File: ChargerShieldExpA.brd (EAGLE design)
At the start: 160 x 99.1 mm, 101 parts, among them IC1 TL431, IC2 LM324N, Q1 BUZ11, Q2 BD648, Q3 BUZ171, Q4 IRFZ48Z, T1 BC548, X1 +Vin, X2 VCC, X3 Battery

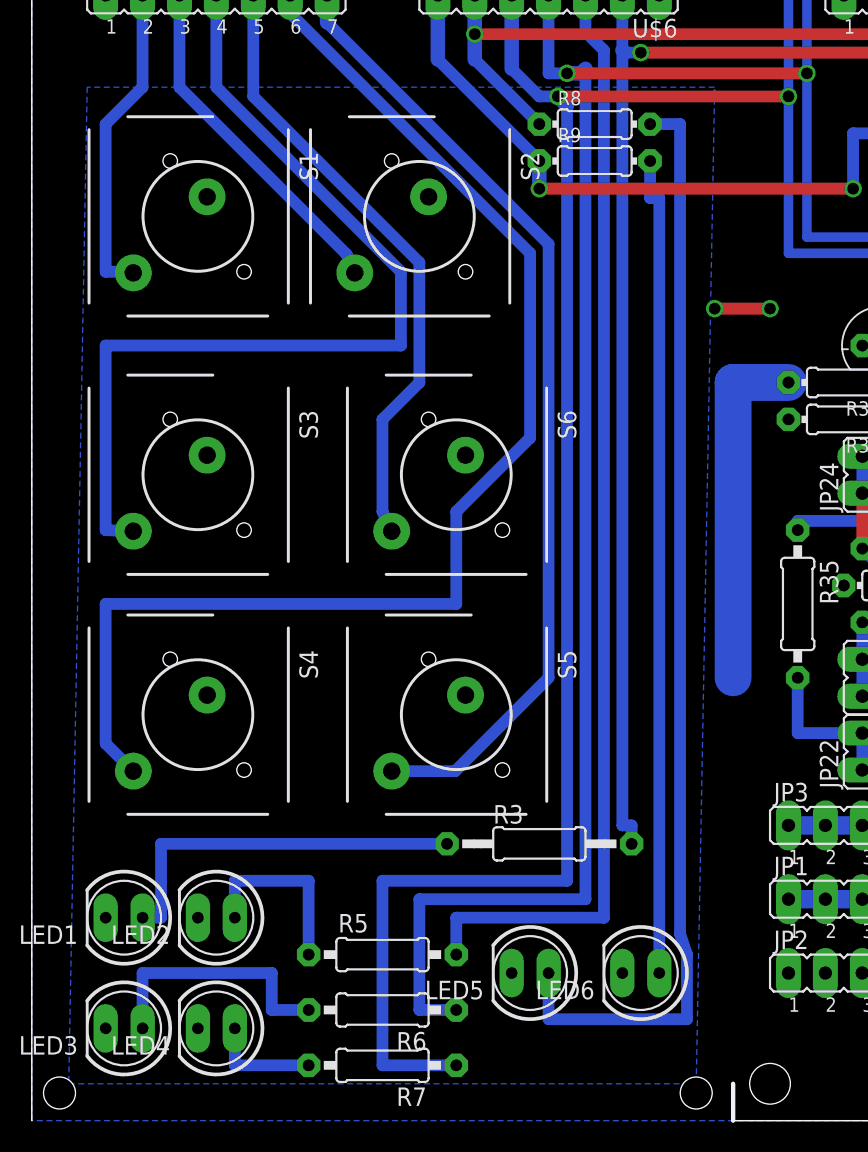
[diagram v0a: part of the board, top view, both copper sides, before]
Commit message: update
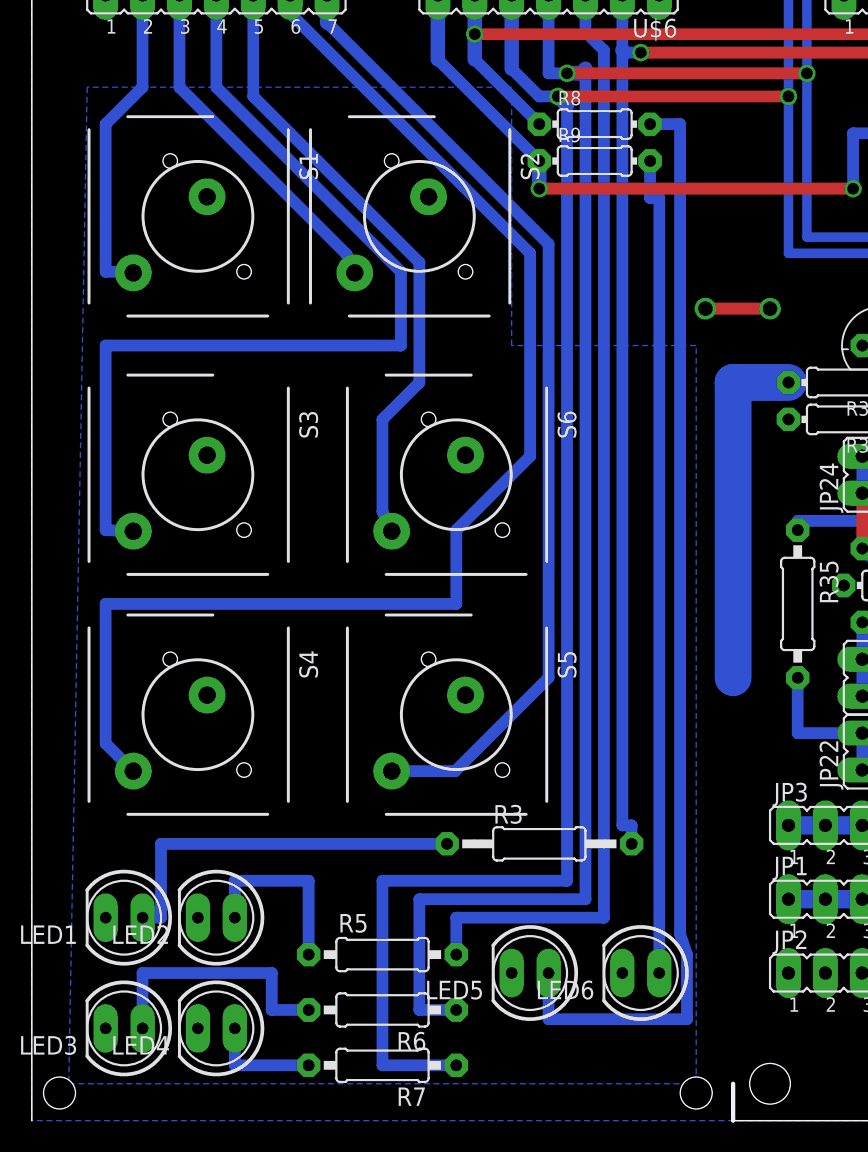
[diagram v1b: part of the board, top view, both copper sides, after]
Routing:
- net GND: track 168.7 -> 169.3 mm
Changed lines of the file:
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@@
 <setting verticaltext="up"/>
 </settings>
-<grid distance="1.27" unitdist="mm" unit="mm" style="lines" multiple="2" display="yes" altdistance="0.15875" altunitdist="mm" altunit="mm"/>
+<grid distance="0.05" unitdist="inch" unit="mm" style="lines" multiple="1" display="yes" altdistance="0.025" altunitdist="inch" altunit="mm"/>
 <layers>
 <layer number="1" name="Top" color="4" fill="1" visible="yes" active="yes"/>
@@
 <wire x1="19.05" y1="11.43" x2="19.05" y2="-3.81" width="0.8128" layer="1" style="shortdash"/>
 <contactref element="JP20" pad="3"/>
-<via x="5.08" y="38.1" extent="1-16" drill="0.8" shape="square"/>
+<via x="5.08" y="38.1" extent="1-16" drill="1" shape="square"/>
 <wire x1="22.86" y1="-7.62" x2="22.86" y2="-11.47" width="1.6764" layer="16"/>
 <wire x1="22.86" y1="-11.47" x2="22.82" y2="-10.16" width="1.6764" layer="16"/>
@@
 <contactref element="S4" pad="1"/>
 <contactref element="S5" pad="1"/>
-<via x="1.27" y="38.1" extent="1-16" drill="0.8" shape="square"/>
-<wire x1="1.27" y1="38.1" x2="5.08" y2="38.1" width="0.8128" layer="1"/>
+<via x="0.635" y="38.1" extent="1-16" drill="1" shape="square"/>
+<wire x1="0.635" y1="38.1" x2="5.08" y2="38.1" width="0.8128" layer="1"/>
 <wire x1="2.54" y1="33.02" x2="2.54" y2="12.7" width="2.54" layer="16"/>
 <wire x1="2.54" y1="33.02" x2="6.35" y2="33.02" width="2.54" layer="16"/>
@@
 <polygon width="1.27" layer="16" isolate="0.6096" orphans="yes">
 <vertex x="0" y="-15.24"/>
-<vertex x="1.27" y="53.34"/>
+<vertex x="0" y="35.56"/>
+<vertex x="-12.7" y="35.56"/>
+<vertex x="-12.7" y="53.34"/>
 <vertex x="-41.91" y="53.34"/>
 <vertex x="-43.18" y="-15.24"/>
@@
 <wire x1="-27.94" y1="59.69" x2="-27.94" y2="58.42" width="0.8128" layer="16"/>
 <wire x1="-27.94" y1="58.42" x2="-11.43" y2="41.91" width="0.8128" layer="16"/>
-<wire x1="-11.43" y1="41.91" x2="-11.43" y2="29.21" width="0.8128" layer="16"/>
+<wire x1="-11.43" y1="41.91" x2="-11.43" y2="27.94" width="0.8128" layer="16"/>
 <wire x1="-40.64" y1="17.78" x2="-40.64" y2="8.1788" width="0.8128" layer="16"/>
 <wire x1="-40.64" y1="8.1788" x2="-38.735" y2="6.2738" width="0.8128" layer="16"/>
-<wire x1="-11.43" y1="29.21" x2="-16.51" y2="24.13" width="0.8128" layer="16"/>
-<wire x1="-16.51" y1="24.13" x2="-16.51" y2="17.78" width="0.8128" layer="16"/>
+<wire x1="-11.43" y1="27.94" x2="-16.51" y2="22.86" width="0.8128" layer="16"/>
+<wire x1="-16.51" y1="22.86" x2="-16.51" y2="17.78" width="0.8128" layer="16"/>
 <wire x1="-16.51" y1="17.78" x2="-40.64" y2="17.78" width="0.8128" layer="16"/>
 <contactref element="U$3" pad="6"/>
